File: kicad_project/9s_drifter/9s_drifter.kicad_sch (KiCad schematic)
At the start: 8 parts, among them SW1 SW_Reed

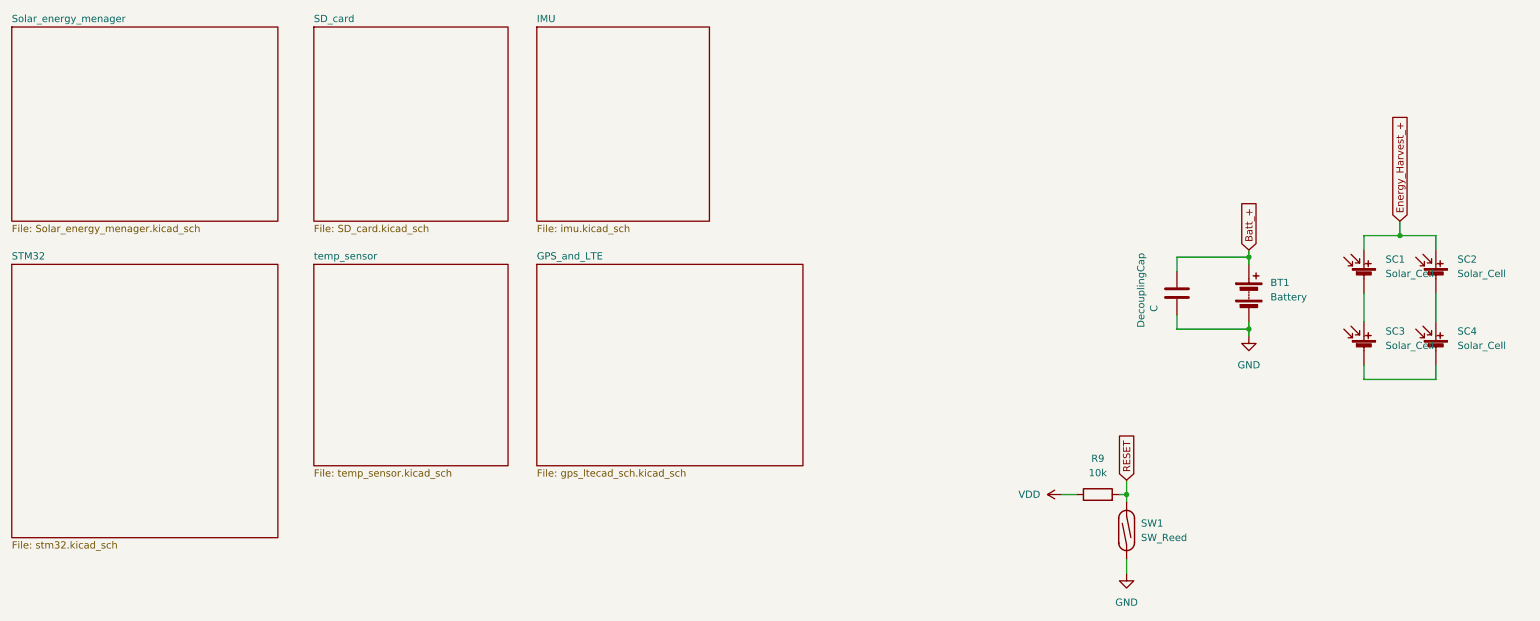
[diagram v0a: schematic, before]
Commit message: Update
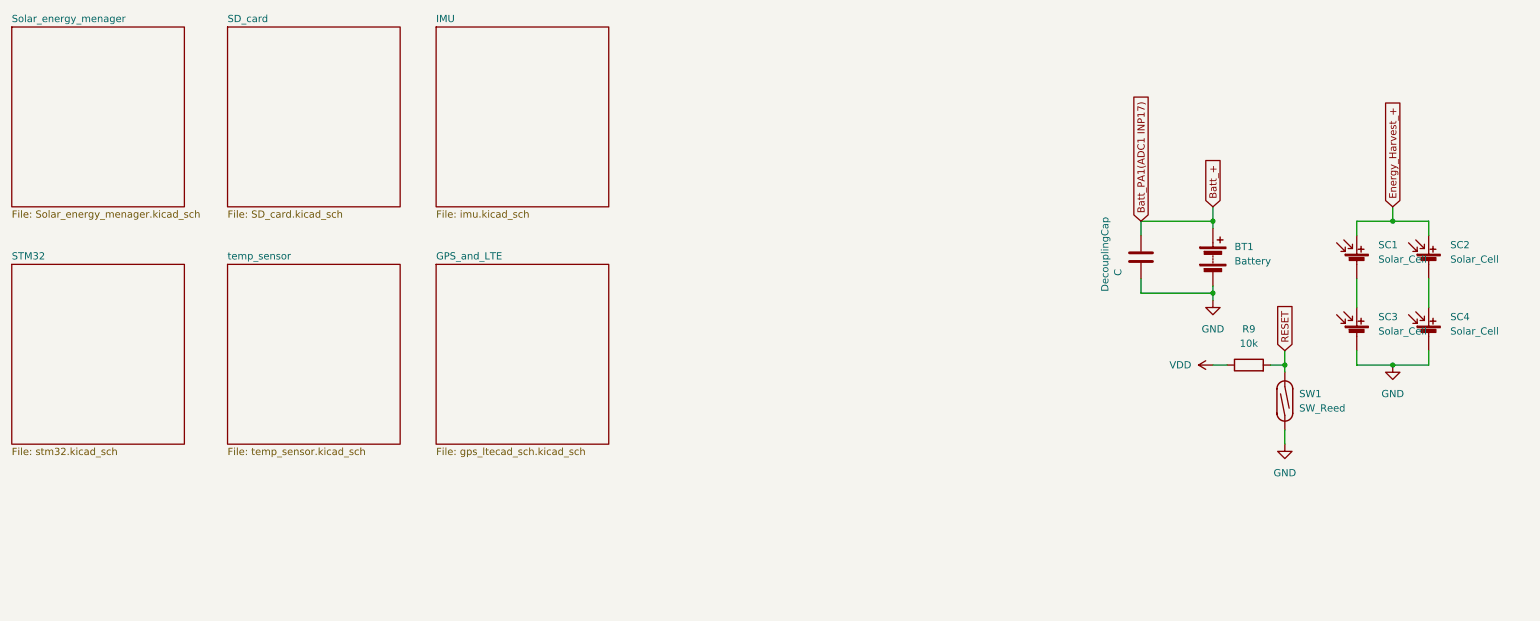
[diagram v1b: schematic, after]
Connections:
- net GND: now also SC3.2 (-), SC4.2 (-)
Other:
- moved on the sheet: BT1, DecouplingCap, R9, SC1, SC2, SC3, SC4, SW1
